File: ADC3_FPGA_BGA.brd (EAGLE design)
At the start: 40.4 x 44.4 mm, 114 parts, among them CON1 MEZZANINE_2X30, CON2 MEZZANINE_2X30, CON3 USB-SC, IC1 ARTIX7-FTG256, IC2 3.3V, IC3 2.5V, IC4 MPM3804, IC5 MPM3804, IC6 EEPROM, IC7 93LC56, IC8 FT2232H, IC9 HyperRAM, J1 BANK34, J2 BANK35, J3 25M, X1 25MHz, X2 12MHz

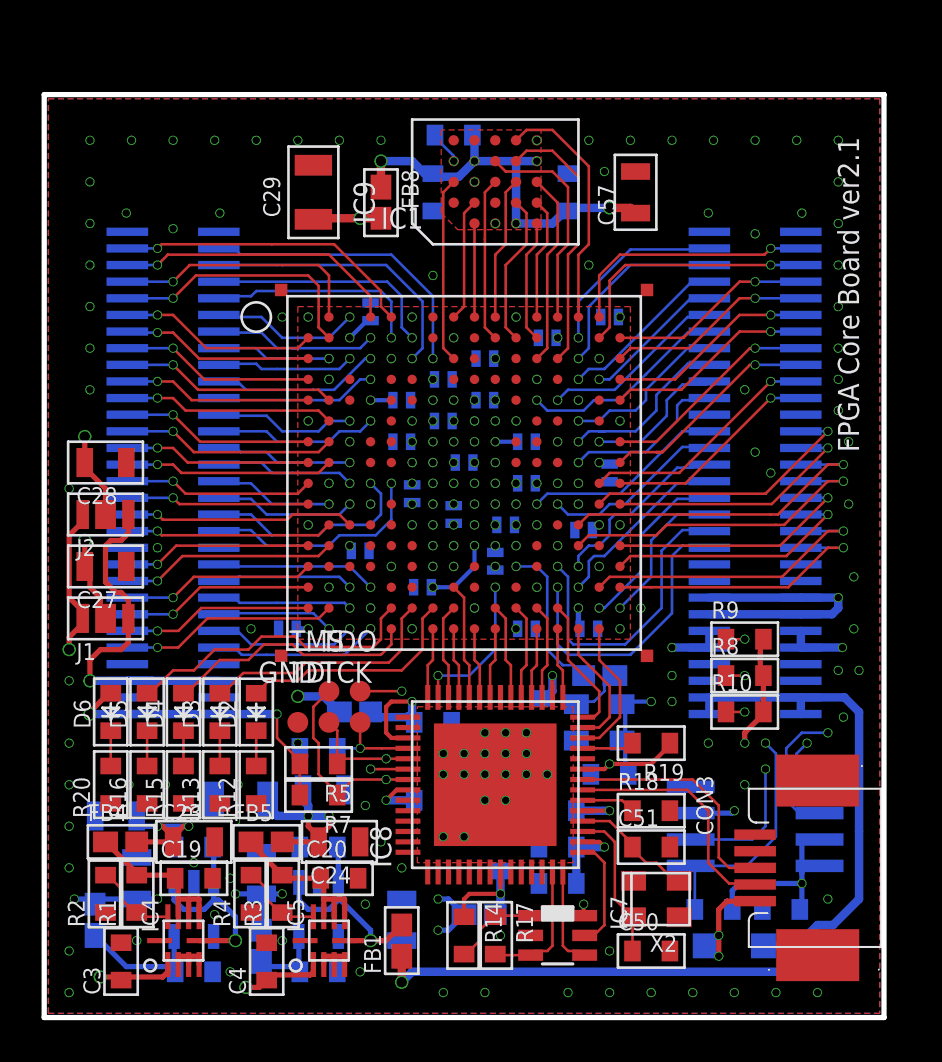
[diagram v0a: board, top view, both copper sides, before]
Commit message: Type-C
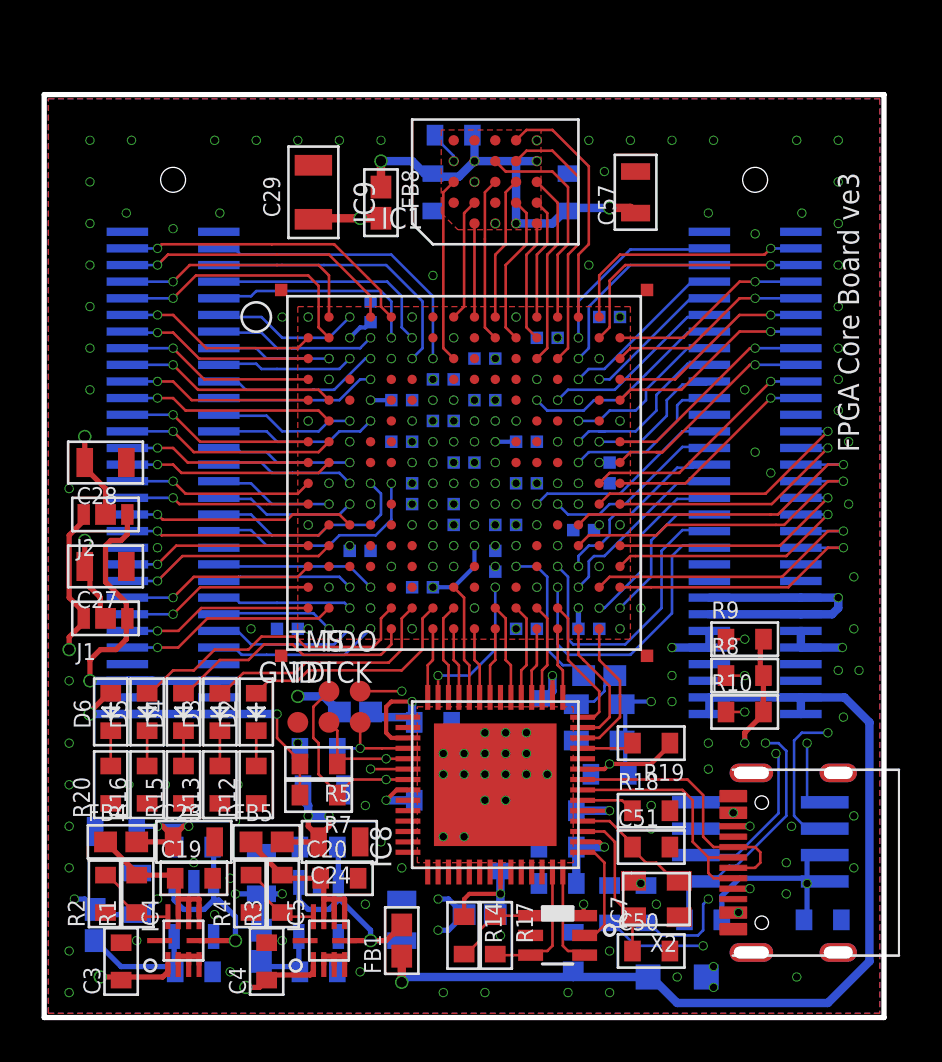
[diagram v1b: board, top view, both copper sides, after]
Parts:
- removed C30: 10u, my_rcl:3216
- added R22, R23: 5.1k, my_rcl:1608
- C1, C10, C17, C18, C19, C20, C3, C4, C44, C45, C46, C47, C48, C49, C50, C51, C52, C53, C54, C55, C56, C9: device my_rcl:1608 -> my_rcl:1608C
- CON3: value USB-SC -> USB-C; device my_connector:UX60SC-MB-5ST -> my_connector:5077CR-16-SMC2-BK-TR
- J1, J2: device my_rcl:2012-3-J -> my_rcl:1608-3-J
- TP1, TP2, TP3, TP4, TP5: device my_connector:TESTPAD -> my_connector:TESTPAD-SMALL
- moved C1 11.8 mm to (5.25, -23.0), turned to 90 degrees
- moved D1 3.13 mm to (10.2, -24.2), turned to 0 degrees
- moved CON3 3.01 mm to (13.2, -18.8), turned to 90 degrees
- moved C44 2.06 mm to (17.2, -21.5), turned to 180 degrees
- moved IC6 0.79 mm to (14.2, -17.8)
- moved C22 0.75 mm to (-15.8, -20.2)
- moved C25 0.75 mm to (-16.8, -17.2)
- moved R11 0.71 mm to (11.5, -21.5)
- moved FB3 0.25 mm to (-17.8, -21.8)
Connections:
- new net N$6: CON3.A5:CC1, R22.2
- new net N$7: CON3.B5:CC2, R23.2
- net +1V0: no longer C30.1
- net GND: now also CON3.A1,B12:GND, CON3.B1,A12:GND, CON3.SHILED1, CON3.SHILED2, CON3.SHILED3, CON3.SHILED4, CON3.SHILED5, CON3.SHILED6, CON3.SHILED7, CON3.SHILED8, R22.1, R23.1; no longer C30.2, CON3.5, CON3.M1, CON3.M2
- net USB_+5V: now also CON3.A4,B9:VBUS, CON3.B4,A9:VBUS; no longer CON3.1
- net USB_DM: now also CON3.A7:DN1, CON3.B7:DN2; no longer CON3.2
- net USB_DP: now also CON3.A6:DP1, CON3.B6:DP2; no longer CON3.3
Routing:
- net N$7: track 0.00 -> 9.98 mm, vias 0 -> 2
- net N$6: track 0.00 -> 9.88 mm, vias 0 -> 2
- net USB_+5V: track 5.91 -> 9.90 mm, vias 2 -> 4
- net +1V0: track 9.65 -> 6.77 mm
- net VIN: track 45.1 -> 47.1 mm
- net USB_DP: track 11.5 -> 13.1 mm
- net +3V3: track 69.6 -> 70.7 mm
- net FLASH_CS: track 33.9 -> 34.7 mm
- net +1V8: track 36.0 -> 35.3 mm
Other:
- board text added: "FPGA Core Board ve3"
- board text removed: "FPGA Core Board ver2.1"
